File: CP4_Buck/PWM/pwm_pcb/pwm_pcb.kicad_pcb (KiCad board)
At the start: 2 copper layers, 64 x 47 mm, 13 parts, among them J1 in, J2 ref, J3 out, U2 LM324, U3 LTC6702CDC_PBF

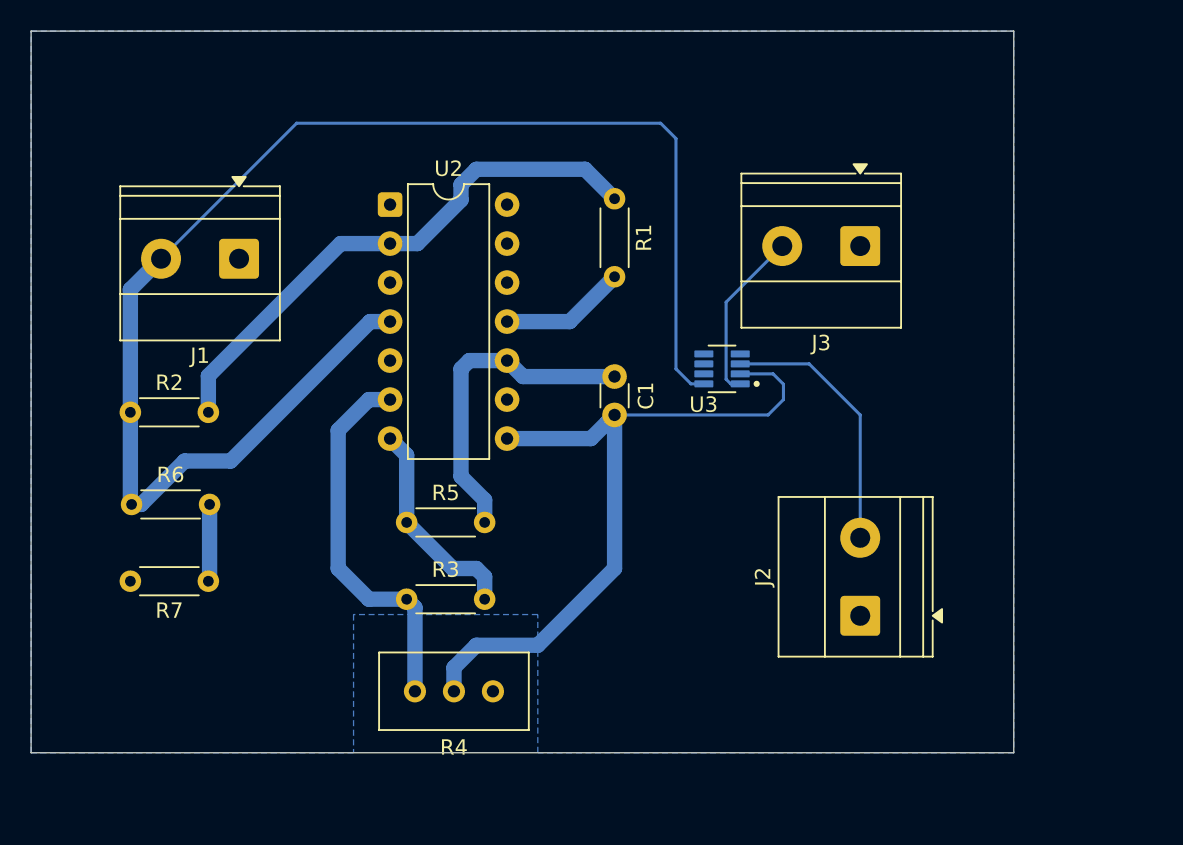
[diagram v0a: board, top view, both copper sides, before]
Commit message: Add files via upload
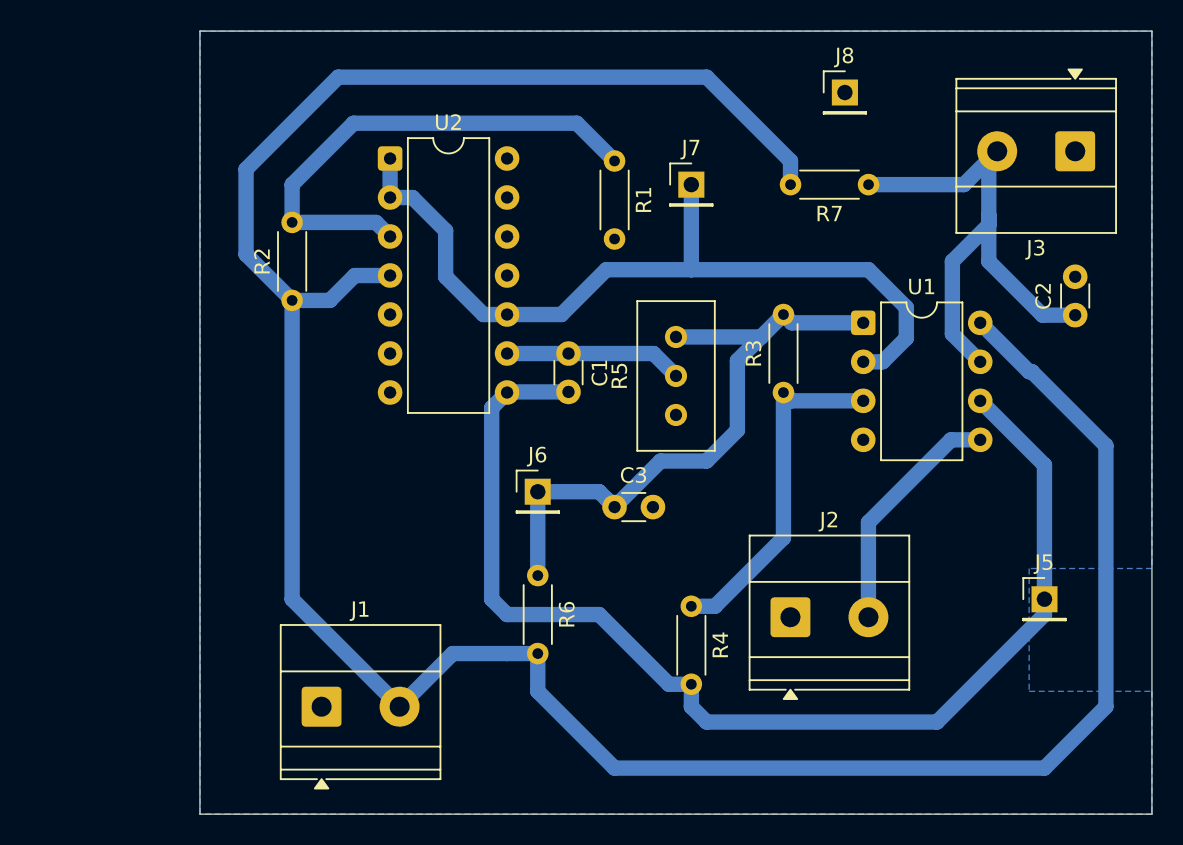
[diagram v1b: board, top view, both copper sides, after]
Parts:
- removed U3: LTC6702CDC_PBF, LTC6702CTS8_TRMPBF:SOT65P280X100-8N
- added C2: 1.8p, Capacitor_THT:C_Disc_D3.0mm_W1.6mm_P2.50mm, F.Cu at (175.0, 88.5)
- added C3: 1.8p, Capacitor_THT:C_Disc_D3.0mm_W1.6mm_P2.50mm, F.Cu at (145.0, 101.0)
- added J5: Vb_pin, Connector_PinHeader_2.54mm:PinHeader_1x01_P2.54mm_Vertical, F.Cu at (173.0, 107.0)
- added J6: Va_pin, Connector_PinHeader_2.54mm:PinHeader_1x01_P2.54mm_Vertical, F.Cu at (140.0, 100.0)
- added J7: Vref_pin, Connector_PinHeader_2.54mm:PinHeader_1x01_P2.54mm_Vertical, F.Cu at (150.0, 80.0)
- added J8: gnd_pin, Connector_PinHeader_2.54mm:PinHeader_1x01_P2.54mm_Vertical, F.Cu at (160.0, 74.0)
- added U1: LM393, Package_DIP:DIP-8_W7.62mm, F.Cu at (161.2, 89.0)
- R4: footprint Potentiometer_THT:Potentiometer_Bourns_3296W_Vertical -> Resistor_THT:R_Axial_DIN0204_L3.6mm_D1.6mm_P5.08mm_Horizontal
- R5: footprint Resistor_THT:R_Axial_DIN0204_L3.6mm_D1.6mm_P5.08mm_Horizontal -> Potentiometer_THT:Potentiometer_Bourns_3296W_Vertical
- R6, R7: value 100k -> 12k
- moved R7 50.2 mm to (161.5, 80.0)
- moved J1 29.7 mm to (125.9, 114.0), turned to 0 degrees
- moved R3 28.0 mm to (156.0, 93.5), turned to 90 degrees
- moved R6 26.9 mm to (140.0, 105.5), turned to -90 degrees
- moved R5 21.3 mm to (149.0, 89.9), turned to 90 degrees
- moved R4 18.8 mm to (150.0, 107.5), turned to -90 degrees
- moved J3 15.3 mm to (175.0, 77.8)
- moved R2 12.8 mm to (124.0, 87.5), turned to 90 degrees
- moved J2 4.55 mm to (156.5, 108.2), turned to 0 degrees
- moved C1 3.35 mm to (142.0, 91.0)
- moved U2 3.00 mm to (130.4, 78.3)
- moved R1 2.46 mm to (145.0, 78.5)
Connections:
- C1 pad 1: Net-(U2C-+) -> Net-(U2C--)
- R1 pad 1: Net-(U2A--) -> Net-(U2A-+)
- R2 pad 2: Net-(U2A--) -> Net-(U2A-+)
- R3 pad 1: Net-(U2B--) -> Net-(U1A-+)
- R4 pad 1: Net-(U2B--) -> Net-(U1A-+)
- R5 pad 2: Net-(U2C-+) -> Net-(U2C--)
- R6 pad 1: Vcc -> Va
- R6 pad 2: Net-(R6-Pad2) -> Vcc
- R7 pad 1: Net-(R6-Pad2) -> Vg
- R7 pad 2: GND -> Vcc
- U2 pad 1: Net-(U2A-+) -> Net-(J7-Pin_1)
- U2 pad 10: Net-(U2C-+) -> Net-(J7-Pin_1)
- U2 pad 2: Net-(U2A--) -> Net-(J7-Pin_1)
- U2 pad 5: Net-(U2A-+) -> (no net)
- U2 pad 6: Net-(U2B--) -> (no net)
- U2 pad 7: Va -> (no net)
- U2 pad 9: Net-(U2A-+) -> Net-(U2C--)
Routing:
- net Vcc: track 93.5 -> 170.1 mm
- net Net-(J7-Pin_1): track 0.00 -> 54.3 mm
- net Net-(U2A--): track 36.0 -> 0.00 mm
- net Net-(U2A-+): track 0.00 -> 32.9 mm
- net Vb: track 48.5 -> 76.6 mm
- net Va: track 13.9 -> 41.4 mm
- net Net-(U2B--): track 24.7 -> 0.00 mm
- net Vg: track 11.2 -> 35.0 mm
- net Net-(U1A-+): track 0.00 -> 22.7 mm
- net Net-(U2C-+): track 21.3 -> 0.00 mm
- net Net-(U2C--): track 0.00 -> 11.6 mm
- net GND: track 8.21 -> 0.00 mm
- net Net-(R6-Pad2): track 5.03 -> 0.00 mm
- net Vr: track 17.2 -> 15.7 mm
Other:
- board size 64 x 47 mm -> 62 x 51 mm
